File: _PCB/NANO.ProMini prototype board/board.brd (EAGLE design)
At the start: 93.2 x 100.1 mm, 70 parts, among them T1_5MM 5mm, T2_5MM 5mm, T3_5MM 5mm

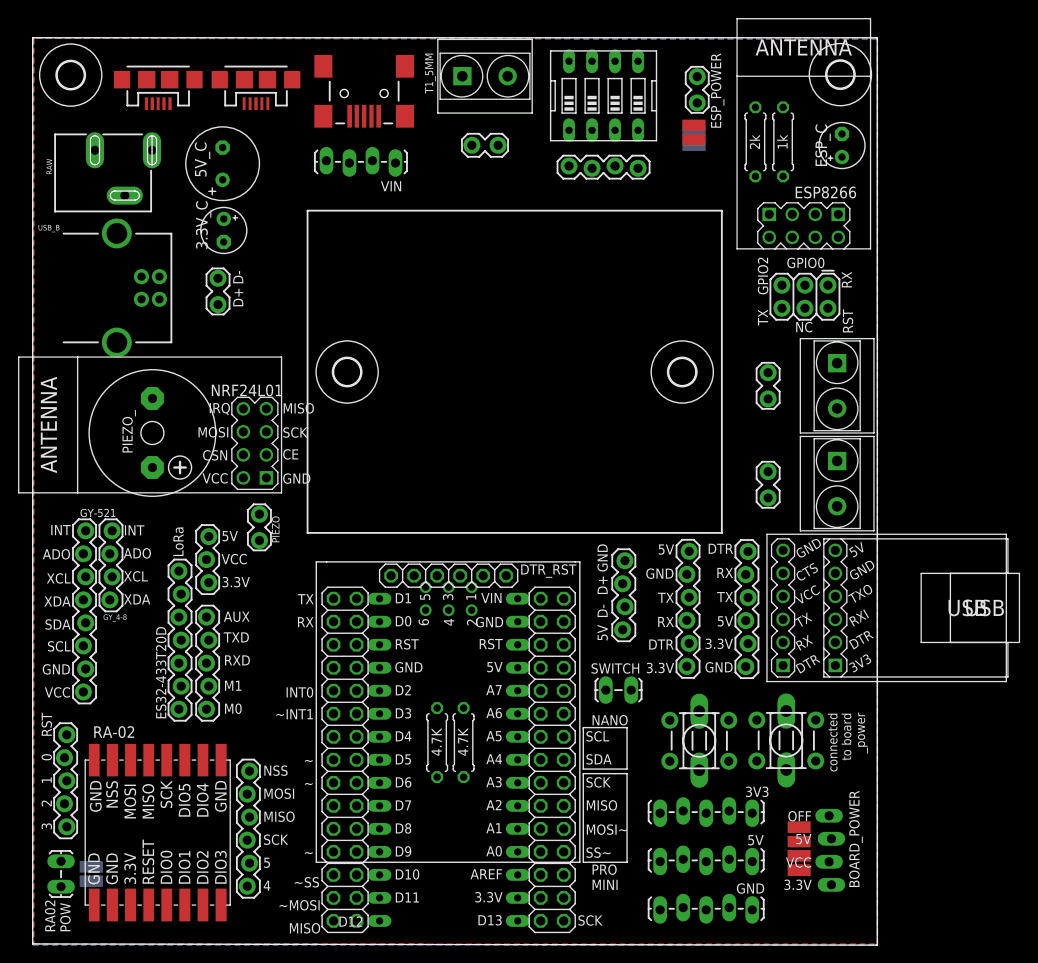
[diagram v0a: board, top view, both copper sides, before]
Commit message: really final prototype
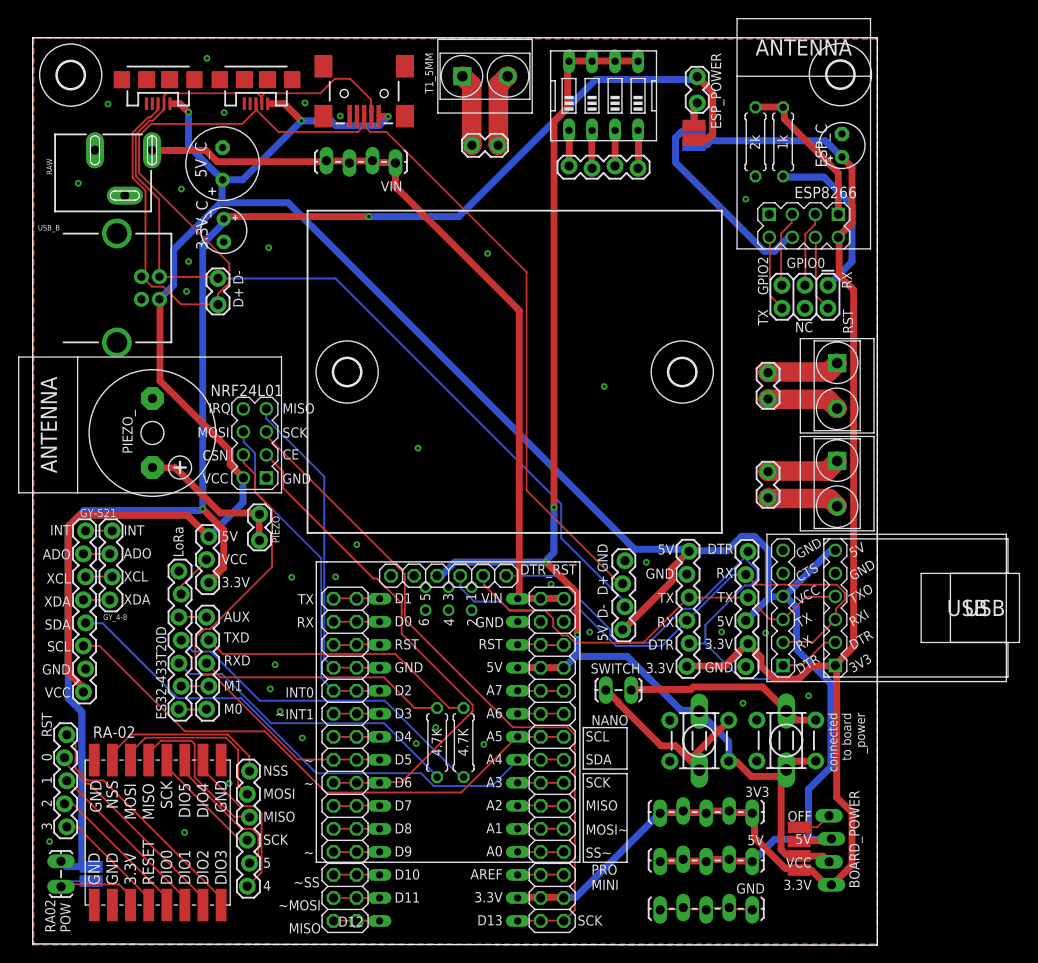
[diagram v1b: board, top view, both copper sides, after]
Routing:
- net 3.3V: track 0.00 -> 342.6 mm, vias 0 -> 2
- net 5V: track 0.00 -> 283.5 mm, vias 0 -> 3
- net D+_5PIN: track 0.00 -> 148.0 mm
- net N$36: track 0.00 -> 144.1 mm, vias 0 -> 3
- net D-_5PIN: track 0.00 -> 119.1 mm
- net VIN: track 0.00 -> 86.6 mm
- net SCK_NRF: track 0.00 -> 77.3 mm
- net N$66: track 0.00 -> 67.4 mm
- net A5: track 0.00 -> 62.3 mm
- net SDA_GY521: track 0.00 -> 61.5 mm
- net N$57: track 0.00 -> 60.8 mm
- net CE_NRF: track 0.00 -> 56.6 mm
- net CSN_NRF: track 0.00 -> 53.3 mm
- net N$62: track 0.00 -> 47.1 mm
- net MOSI_NRF: track 0.00 -> 37.8 mm
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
